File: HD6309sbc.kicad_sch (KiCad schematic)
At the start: 28 parts, among them J1 Conn_01x02_Male, J3 Conn_01x02_Male, SW1 SW_Push, U1 HD63C09, U11 74HC02, U12 74AHC1G08, U13 74HC21D, U14 74HC21D, U15 74HC21D, U4 UM61256FK, U6 28C256, U8 74HC00D

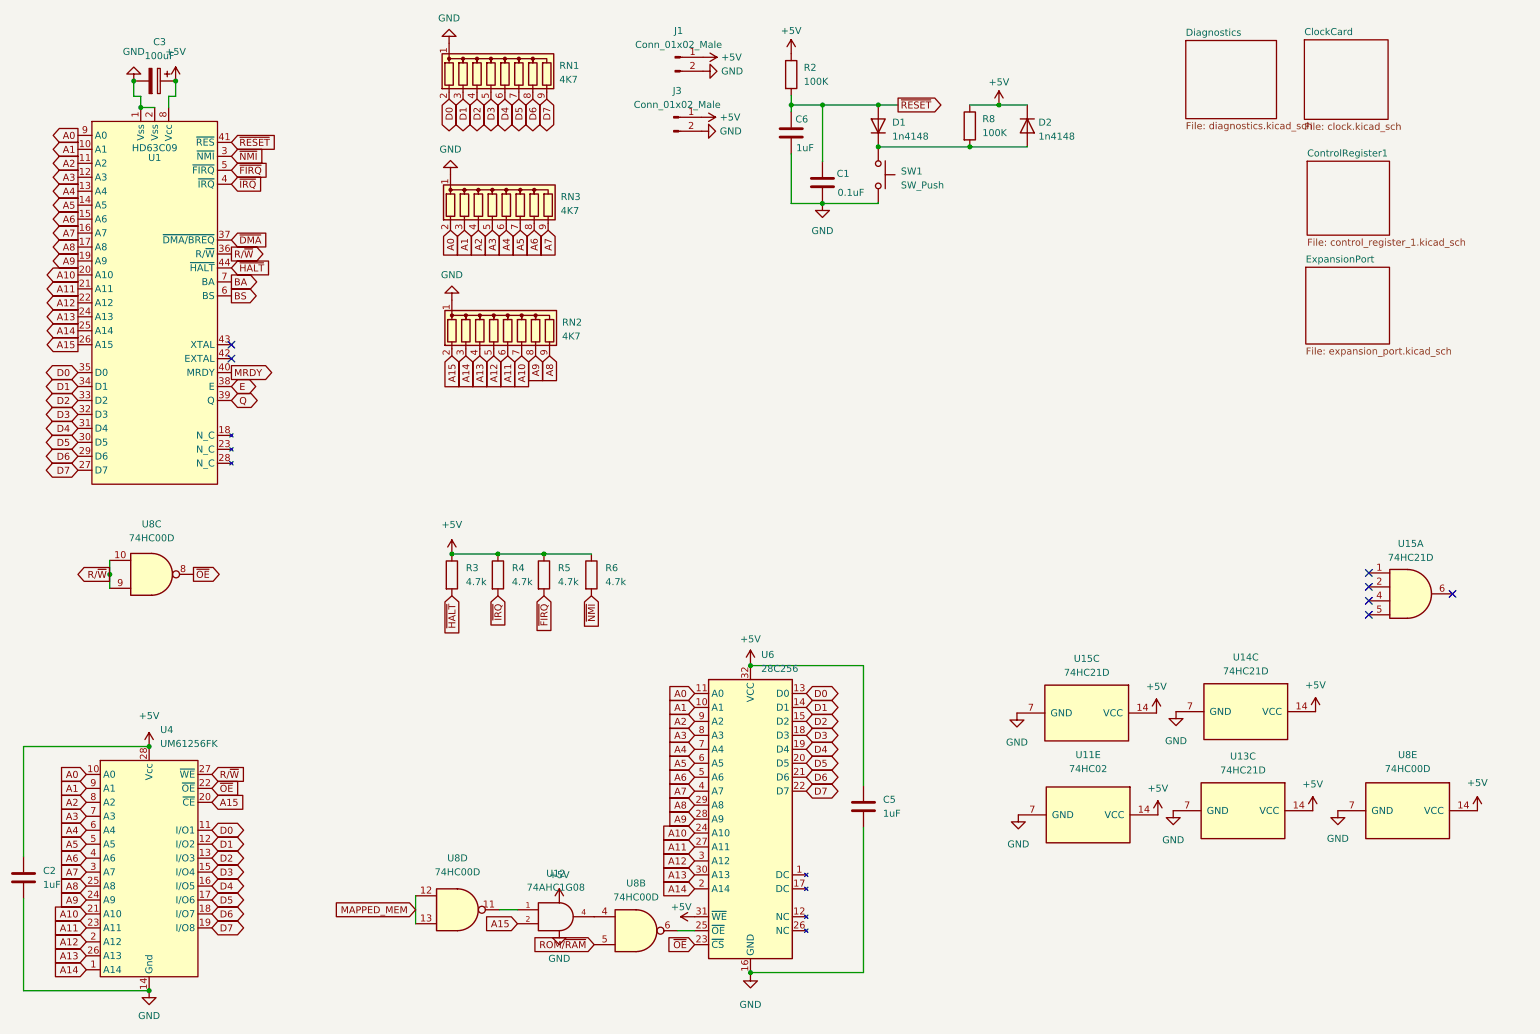
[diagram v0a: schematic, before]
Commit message: convert to new format
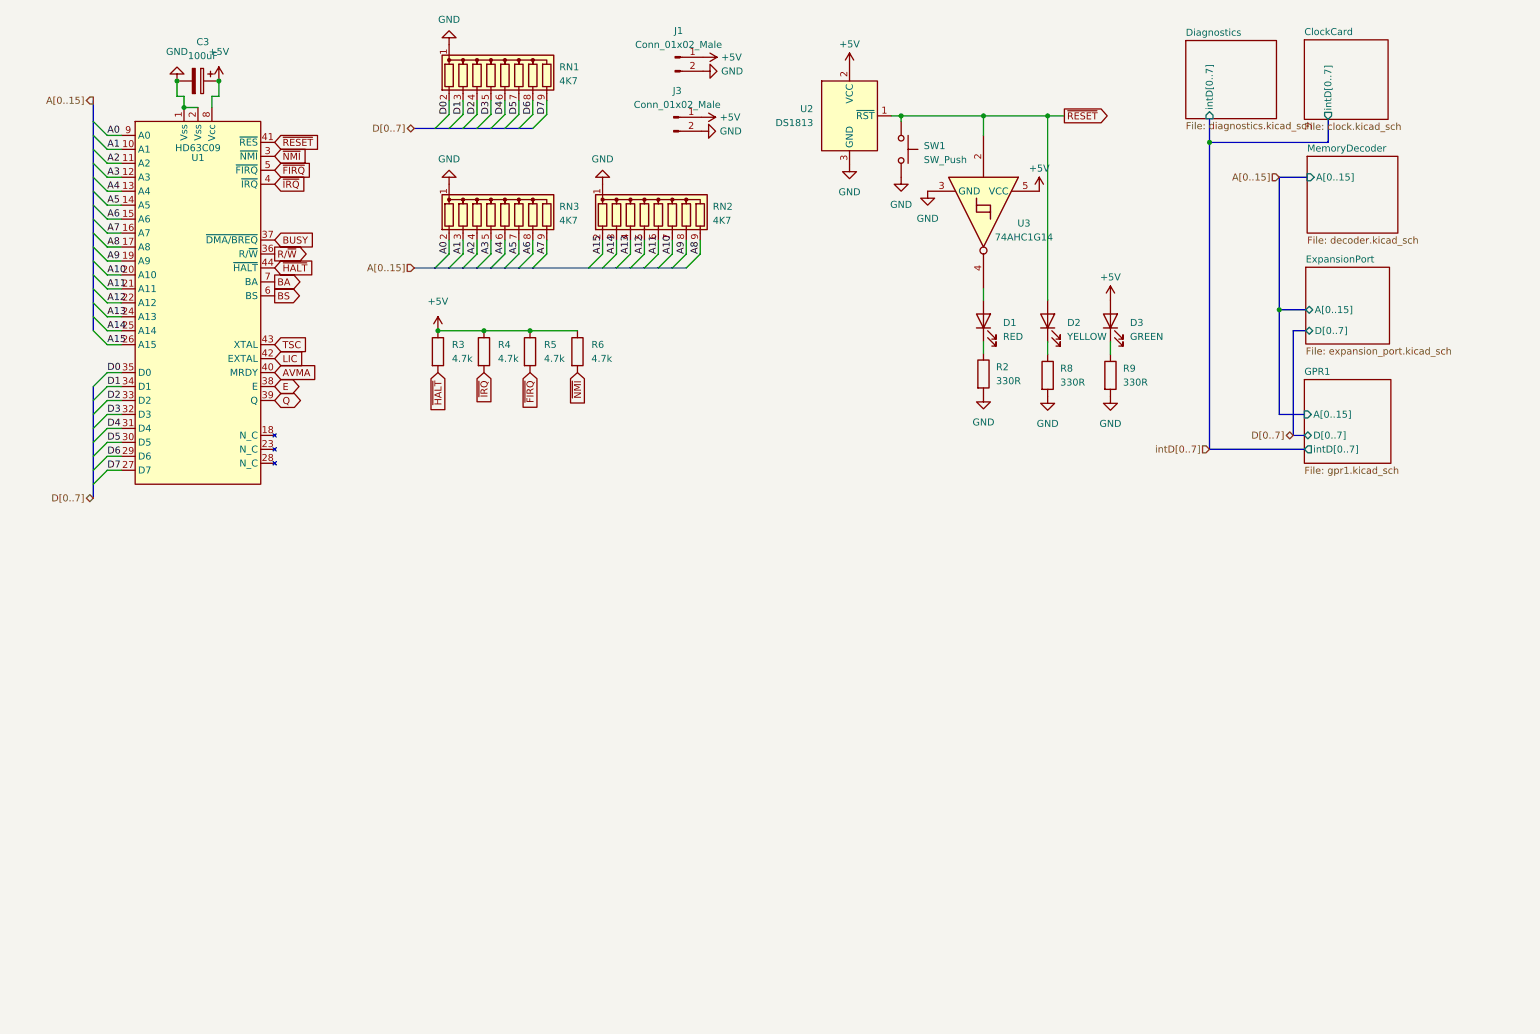
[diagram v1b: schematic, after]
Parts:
- removed C1: 0.1uF, Capacitor_SMD:C_0805_2012Metric_Pad1.18x1.45mm_HandSolder, symbol Device:C
- removed C2, C5, C6: 1uF, Capacitor_SMD:C_0805_2012Metric_Pad1.18x1.45mm_HandSolder, symbol Device:C
- removed D1, D2: 1n4148, Diode_SMD:D_0805_2012Metric_Pad1.15x1.40mm_HandSolder, symbol Device:D
- removed U11: 74HC02, Package_SO:SO-14_3.9x8.65mm_P1.27mm, symbol 74xx:74LS02
- removed U12: 74AHC1G08, Package_SO:TSOP-5_1.65x3.05mm_P0.95mm, symbol 74xGxx:74AHC1G08
- removed U13, U14, U15: 74HC21D, Package_SO:SOIC-14_3.9x8.7mm_P1.27mm, symbol 74xx:74LS21
- removed U4: UM61256FK, Package_DIP:DIP-28_W7.62mm, symbol 6309sbc:UM61256FK
- removed U6: 28C256, Package_LCC:PLCC-32_THT-Socket, symbol 6309sbc:28C256plcc
- removed U8: 74HC00D, Package_SO:SOIC-14_3.9x8.7mm_P1.27mm, symbol 74xx:74HC00
- added D1: RED, LED_SMD:LED_0805_2012Metric_Pad1.15x1.40mm_HandSolder, symbol Device:LED
- added D2: YELLOW, LED_SMD:LED_0805_2012Metric_Pad1.15x1.40mm_HandSolder, symbol Device:LED
- added D3: GREEN, LED_SMD:LED_0805_2012Metric_Pad1.15x1.40mm_HandSolder, symbol Device:LED
- added R9: 330R, Resistor_SMD:R_0805_2012Metric_Pad1.20x1.40mm_HandSolder, symbol Device:R
- added U2: DS1813, Package_TO_SOT_SMD:SOT-23-3, symbol 6309sbc:DS1813
- added U3: 74AHC1G14, Package_TO_SOT_SMD:SOT-353_SC-70-5_Handsoldering, symbol 74xGxx:74AHC1G14
- R2, R8: value 100K -> 330R
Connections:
- net +5V: now also D3.2 (A), U2.2 (VCC), U3.5 (VCC); no longer R2.1, R8.1
- net GND: now also R2.2, R8.2, R9.2, U2.3 (GND), U3.3 (GND)
- net ~{RESET}: now also SW1.1, D2.2 (A), U2.1 (~{RST}), U3.2; no longer R2.2
- net LIC: now reaches U1.42 (EXTAL)
- net TSC: now reaches U1.43 (XTAL)
- net MRDY renamed AVMA
- net ~{DMA} renamed BUSY
- new net: D3.1 (K), R9.1
- new net: D2.1 (K), R8.1
- new net: D1.1 (K), R2.1
- new net: D1.2 (A), U3.4
- no-connect marks 7 -> 0
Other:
- removed sheet ControlRegister1
- added sheet GPR1 (gpr1.kicad_sch)
- added sheet MemoryDecoder (decoder.kicad_sch)
- sheet ClockCard ports: added intD[0..7]; removed none
- sheet Diagnostics ports: added intD[0..7]; removed none
- sheet ExpansionPort ports: added A[0..15], D[0..7]; removed none
- title: (none) -> HD6309 Homebrew SBC
- moved on the sheet: C3, R2, R3, R4, R5, R6, R8, RN2, RN3, SW1, U1
